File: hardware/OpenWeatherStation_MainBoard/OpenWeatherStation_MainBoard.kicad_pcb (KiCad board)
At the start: 2 copper layers, 50.8 x 101.6 mm, 112 parts, among them J2 Conn_01x05_Pin, J3 RJ45_LED_Shielded, J4 Conn_02x07_Odd_Even, Q1 Q_NMOS_GDS, U1 STM32F107VCTx, U10 TL431DBV, U2 FXPS7115D4, U3 HTU21D, U5 PM8800A, U6 POE13P-33L, U7 USBLC6-4SC6, U8 LAN8742A, U9 TCMT1107, Y1 Crystal

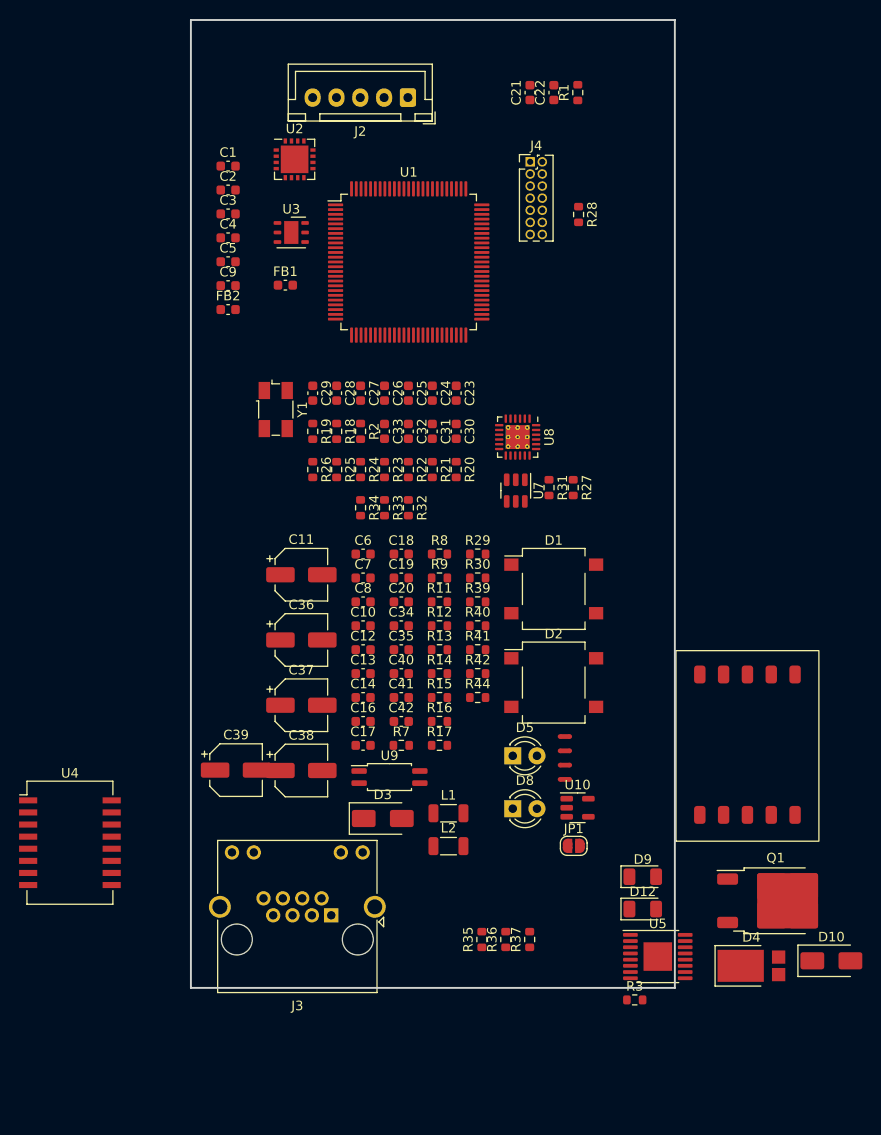
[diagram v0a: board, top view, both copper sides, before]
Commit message: update pcb
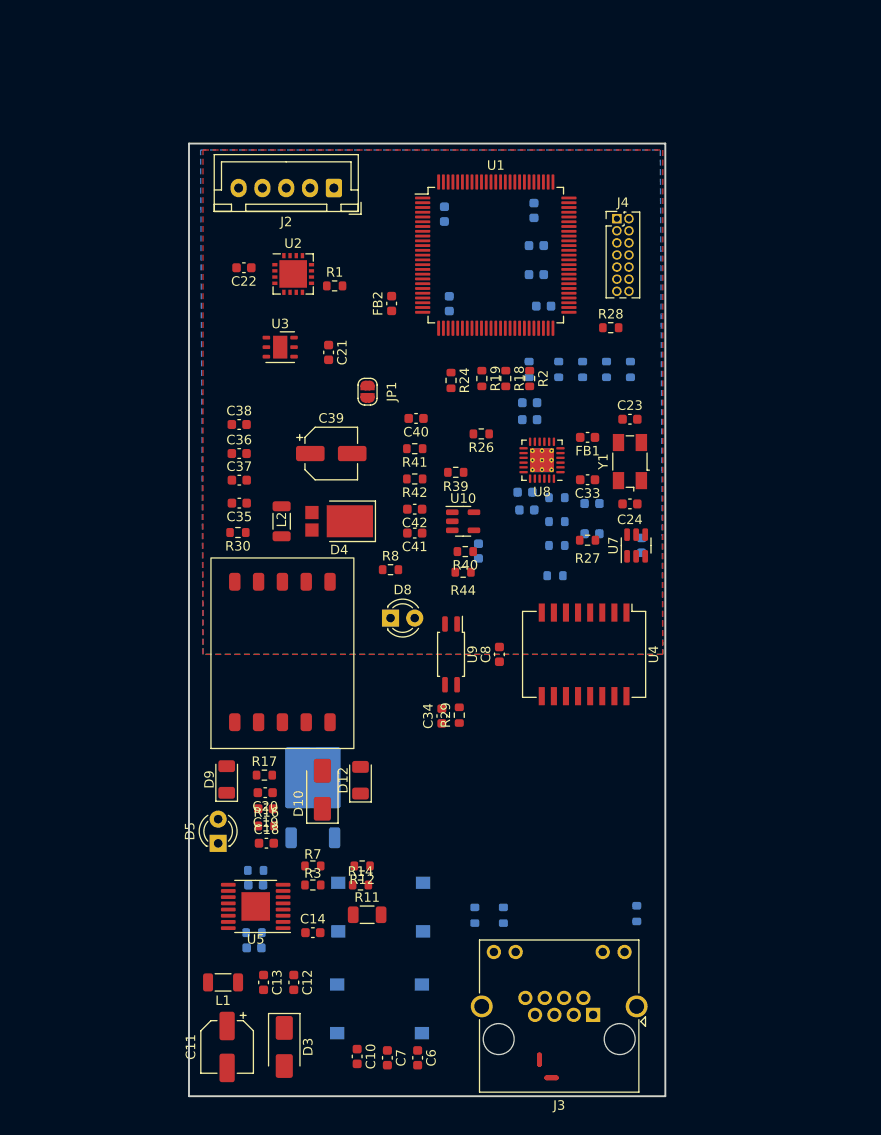
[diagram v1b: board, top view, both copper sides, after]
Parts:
- removed R13: 0.33R, Resistor_SMD:R_0603_1608Metric
- C1, C16, C17, C2, C25, C26, C27, C28, C29, C3, C30, C31, C32, C4, C5, C9, D1, D2, Q1, R15, R20, R21, R22, R23, R25, R31, R32, R33, R34, R35, R36, R37, R9: moved to B.Cu
- C36, C37, C38: footprint Capacitor_SMD:CP_Elec_5x3 -> Capacitor_SMD:C_0603_1608Metric
- R11: footprint Resistor_SMD:R_0603_1608Metric -> Resistor_SMD:R_1206_3216Metric
- moved D4 63.6 mm to (91.8, 128.8), turned to 180 degrees
- moved U4 57.5 mm to (117.5, 142.8), turned to -90 degrees
- moved D10 56.4 mm to (90.0, 157.0), turned to 90 degrees
- moved C6 53.2 mm to (100.0, 185.1), turned to -90 degrees
- moved JP1 52.4 mm to (94.7, 115.2), turned to 90 degrees
- moved C7 50.4 mm to (96.8, 185.1), turned to -90 degrees
- moved C11 50.2 mm to (80.0, 184.0), turned to -90 degrees
- moved Q1 50.0 mm to (89.0, 157.0), turned to 90 degrees
- moved U6 49.8 mm to (85.8, 142.7)
- moved D1 47.7 mm to (96.0, 180.0)
- moved C10 45.2 mm to (93.7, 185.0), turned to -90 degrees
- moved D9 44.9 mm to (80.0, 155.9), turned to 90 degrees
- moved U5 42.5 mm to (83.0, 169.2), turned to 180 degrees
- moved R9 42.0 mm to (82.8, 172.0)
- moved L2 38.3 mm to (85.7, 128.8), turned to -90 degrees
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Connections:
- U5 pad 1: (no net) -> Net-(U5-RT)
- U5 pad 10: (no net) -> Net-(U5-GD)
- U5 pad 11: (no net) -> Net-(D9-K)
- U5 pad 12: (no net) -> Net-(D5-K)
- U5 pad 13: (no net) -> Net-(U5-CS)
- U5 pad 14: (no net) -> Net-(U5-COMP)
- U5 pad 15: (no net) -> GNDA
- U5 pad 16: (no net) -> GNDA
- U5 pad 2: (no net) -> Net-(U5-SS)
- U5 pad 3: (no net) -> unconnected-(U5-AUXII-Pad3)
- U5 pad 4: (no net) -> /PoE/VIN
- U5 pad 5: (no net) -> Net-(U5-RCLASS)
- U5 pad 6: (no net) -> unconnected-(U5-AUXI_IRL-Pad6)
- U5 pad 7: (no net) -> Net-(U5-DCCL)
- U5 pad 8: (no net) -> /PoE/VSS
- U5 pad 9: (no net) -> GNDPWR
- U6 pad 10: (no net) -> Net-(D8-K)
- U6 pad 2: GND -> GNDA
- U6 pad 5: Net-(D4-A) -> (no net)
- U6 pad 6: Net-(D4-A) -> (no net)
- U6 pad 7: Net-(D8-K) -> Net-(D4-A)
- U6 pad 8: Net-(D8-K) -> Net-(D4-A)
- U6 pad 9: (no net) -> Net-(D8-K)
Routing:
- added copper zone on B.Cu, net GND
- added copper zone on F.Cu, net GND
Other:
- board size 50.8 x 101.6 mm -> 50 x 100 mm
